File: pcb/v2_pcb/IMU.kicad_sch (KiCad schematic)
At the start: 13 parts, among them U1000 SCH16T-K01

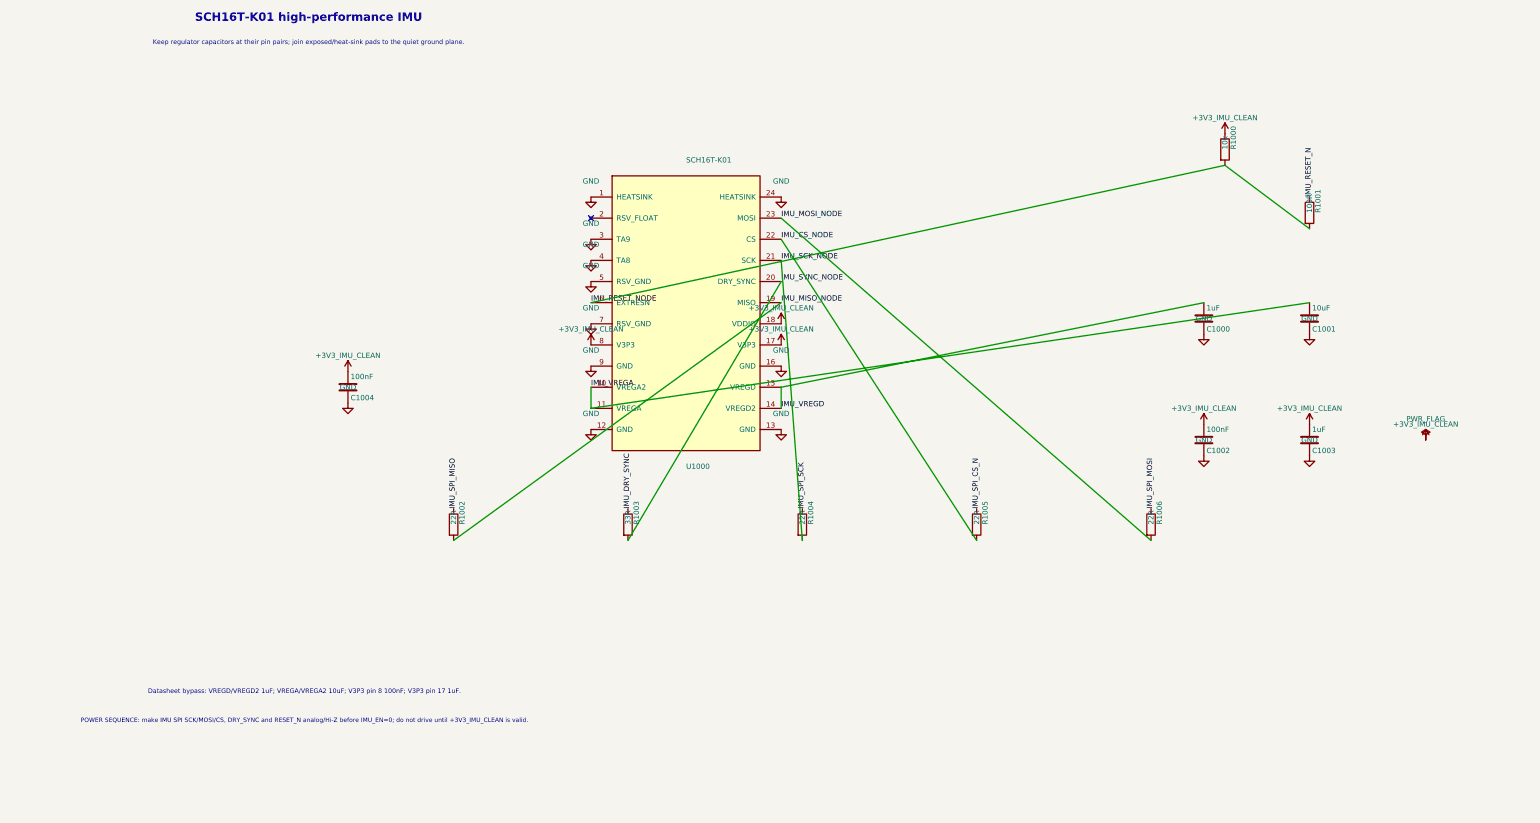
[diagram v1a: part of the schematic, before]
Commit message: clean pcb
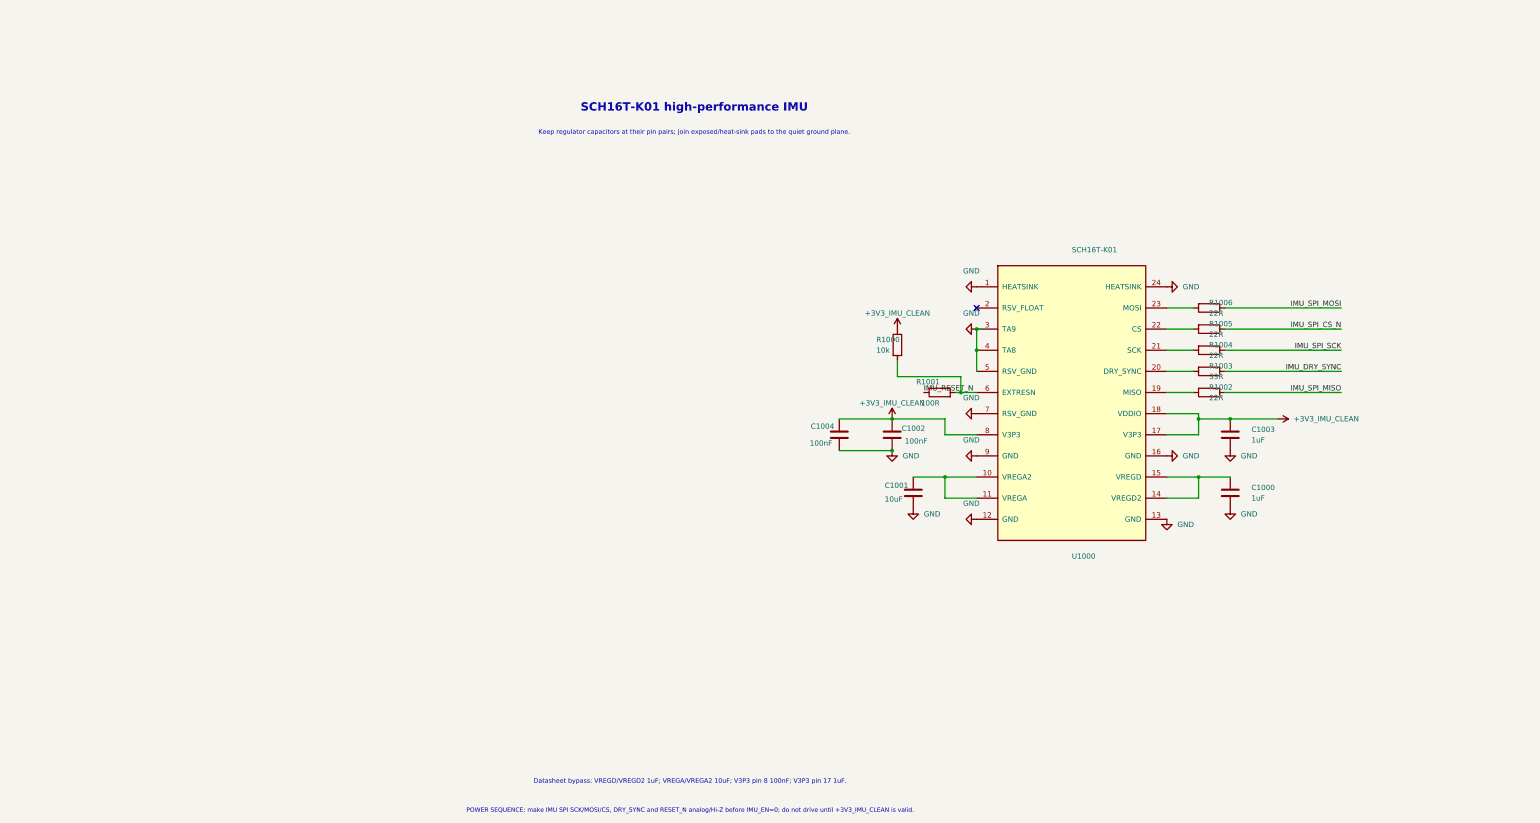
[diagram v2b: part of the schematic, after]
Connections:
- net IMU_CS_NODE: no longer names the net of R1005.2, U1000.22 (CS)
- net IMU_MISO_NODE: no longer names the net of R1002.2, U1000.19 (MISO)
- net IMU_MOSI_NODE: no longer names the net of R1006.2, U1000.23 (MOSI)
- net IMU_RESET_NODE: no longer names the net of R1000.2, R1001.2, U1000.6 (EXTRESN)
- net IMU_SCK_NODE: no longer names the net of R1004.2, U1000.21 (SCK)
- net IMU_SYNC_NODE: no longer names the net of R1003.2, U1000.20 (DRY_SYNC)
- net IMU_VREGA: no longer names the net of C1001.1, U1000.10 (VREGA2), U1000.11 (VREGA)
- net IMU_VREGD: no longer names the net of C1000.1, U1000.14 (VREGD2), U1000.15 (VREGD)
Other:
- moved on the sheet: C1000, C1001, C1002, C1003, C1004, R1000, R1001, R1002, R1003, R1004, R1005, R1006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
